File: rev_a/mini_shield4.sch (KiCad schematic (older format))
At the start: 2 parts

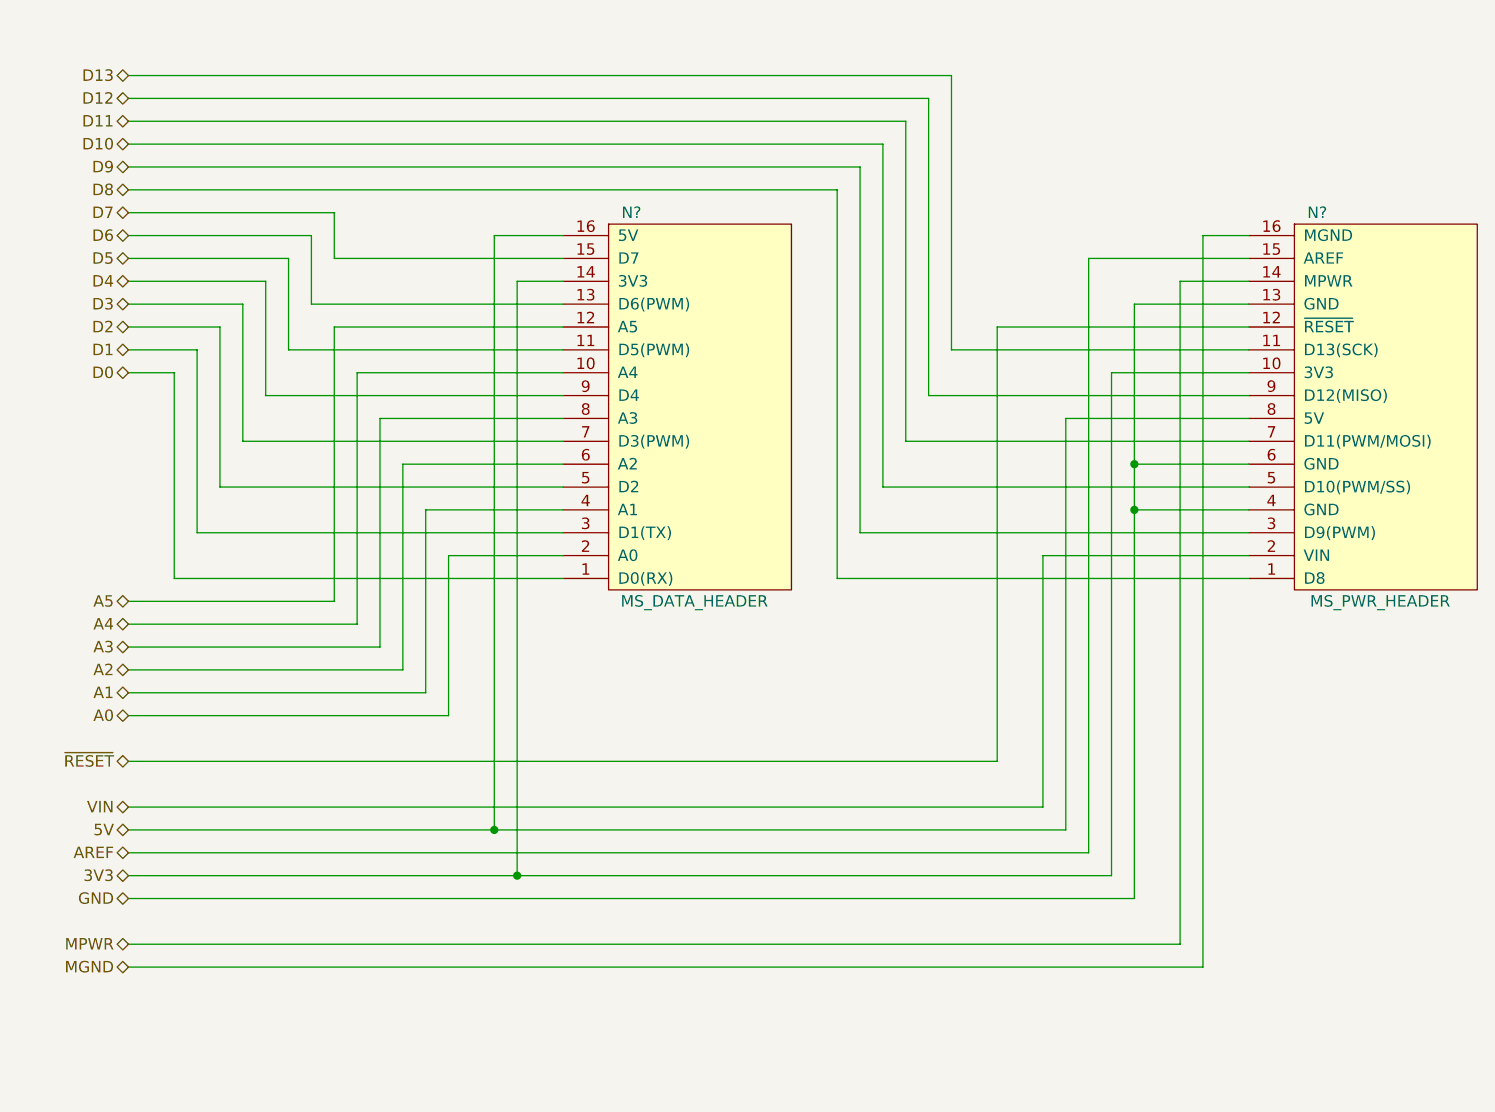
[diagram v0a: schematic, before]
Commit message: Making progress on processor sheet.
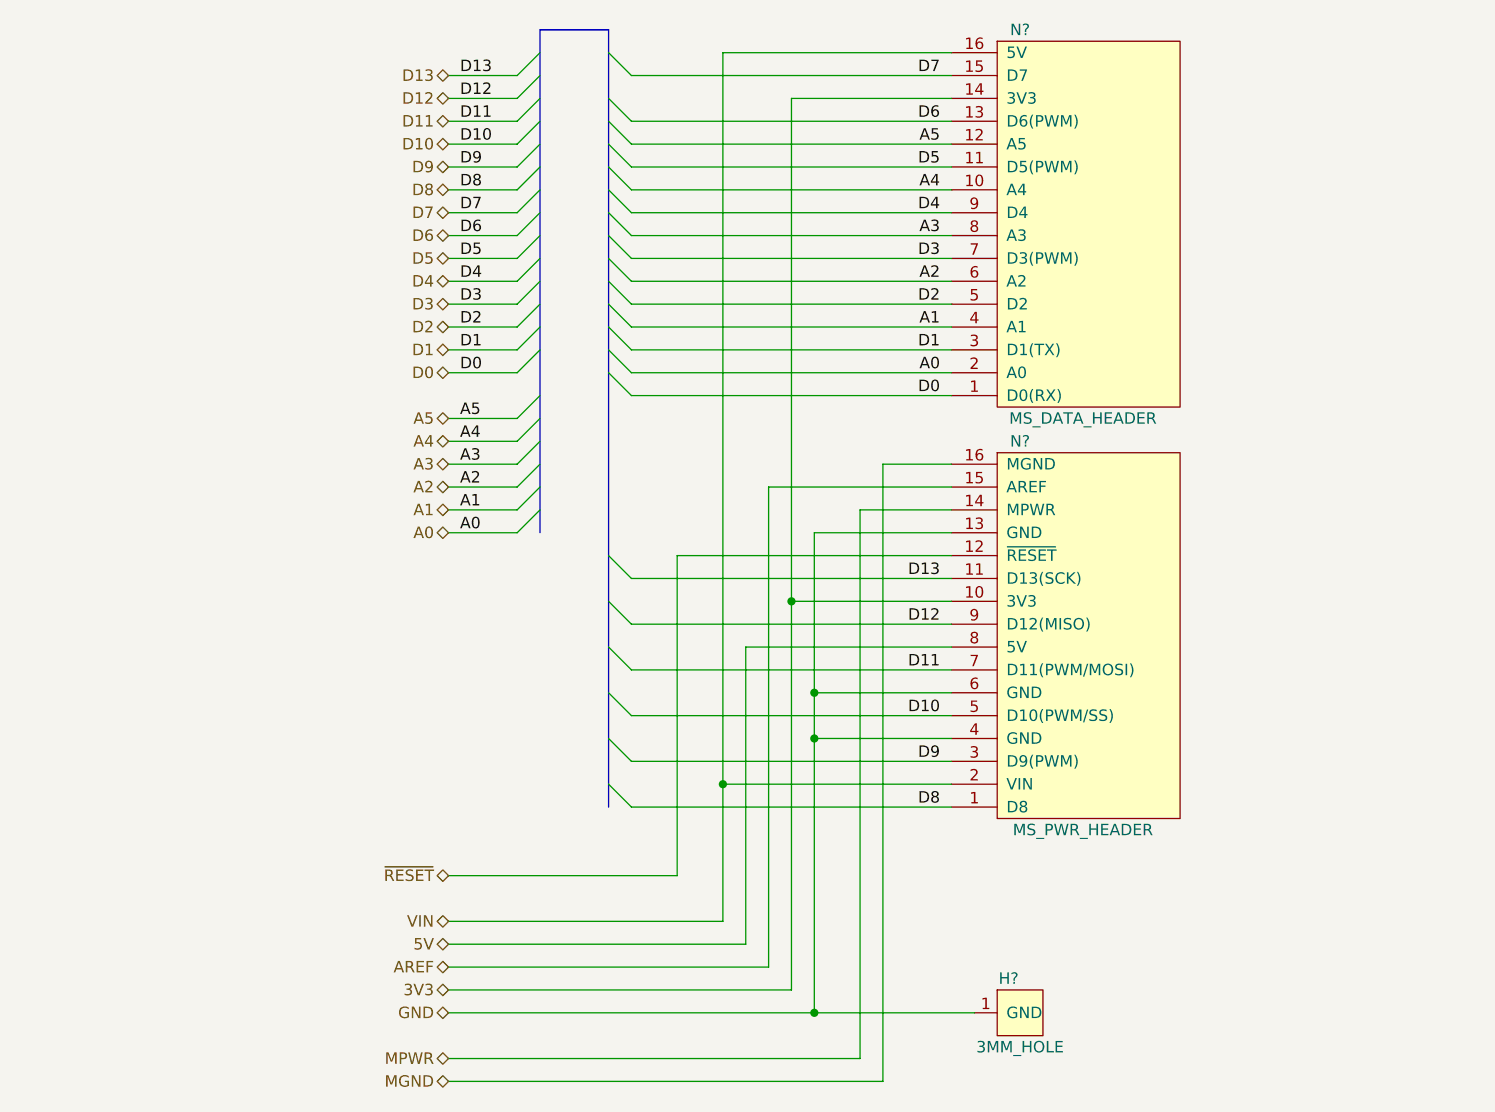
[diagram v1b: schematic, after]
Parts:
- added H?: 3MM_HOLE, symbol 3MM_HOLE
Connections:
- net 5V: no longer N?.16 (5V)
- net GND: now also H?.1 (GND)
- net VIN: now also N?.16 (5V)
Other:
- moved on the sheet: N?
